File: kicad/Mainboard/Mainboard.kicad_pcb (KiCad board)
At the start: 2 copper layers, 46.9 x 107.1 mm, 277 parts, among them J1 ESP8266 module, J10 MIC_EXT, J11 VIB2, J12 SPK_EXT, J13 GPS_CONN, J14 Micro_SD_Card, J15 DBG_CONN, J3 USB_OTG, J4 SWD, J5 BATT, J6 POT_PWR_SW, J7 Conn_01x10, J8 Antenna, J9 VIB1, Q1 BSS138, Q2 BSS138, Q3 BGA6589, Q4 BSS138, Q5 BSS138, Q6 BSS138, Q7 FDV304P, SW1 INT_PTT_SW, T1 AFT05MS004NT1, U1 STM32F777VIT, U10 LM386, U11 LSM9DS1, U13 BGA2874, U2 USBLC6-2SC6, U3 LD1117S50TR_SOT223, U4 LD1117S33TR_SOT223, U5 ADF7021, U6 HMC546MS8GETR, U7 LM2904A, U8 HEF4066B, U9 OPA340UA, X1 12.288MHz

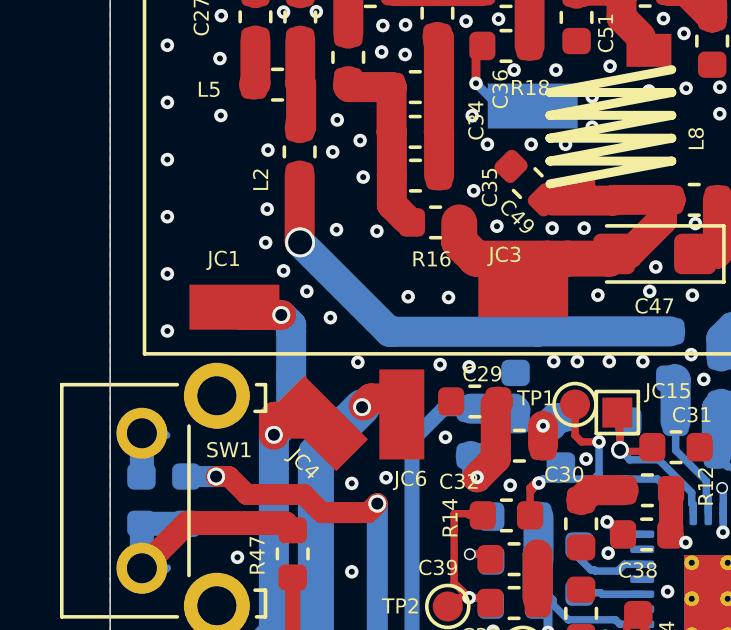
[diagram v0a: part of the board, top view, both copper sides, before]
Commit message: HMI: added design of PCB -> plotted PDF -> plotted production output - Gerbers -> HMI is READY!!
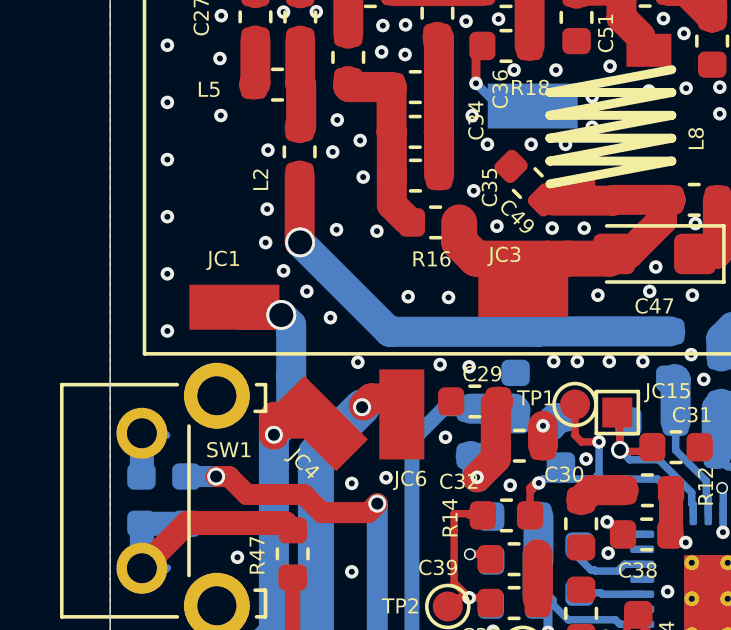
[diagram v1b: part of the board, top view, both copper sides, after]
